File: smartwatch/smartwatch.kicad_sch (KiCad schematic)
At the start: 2 parts, among them U1 ESP32-S3-WROOM-1, U2 AMS1117-3.3

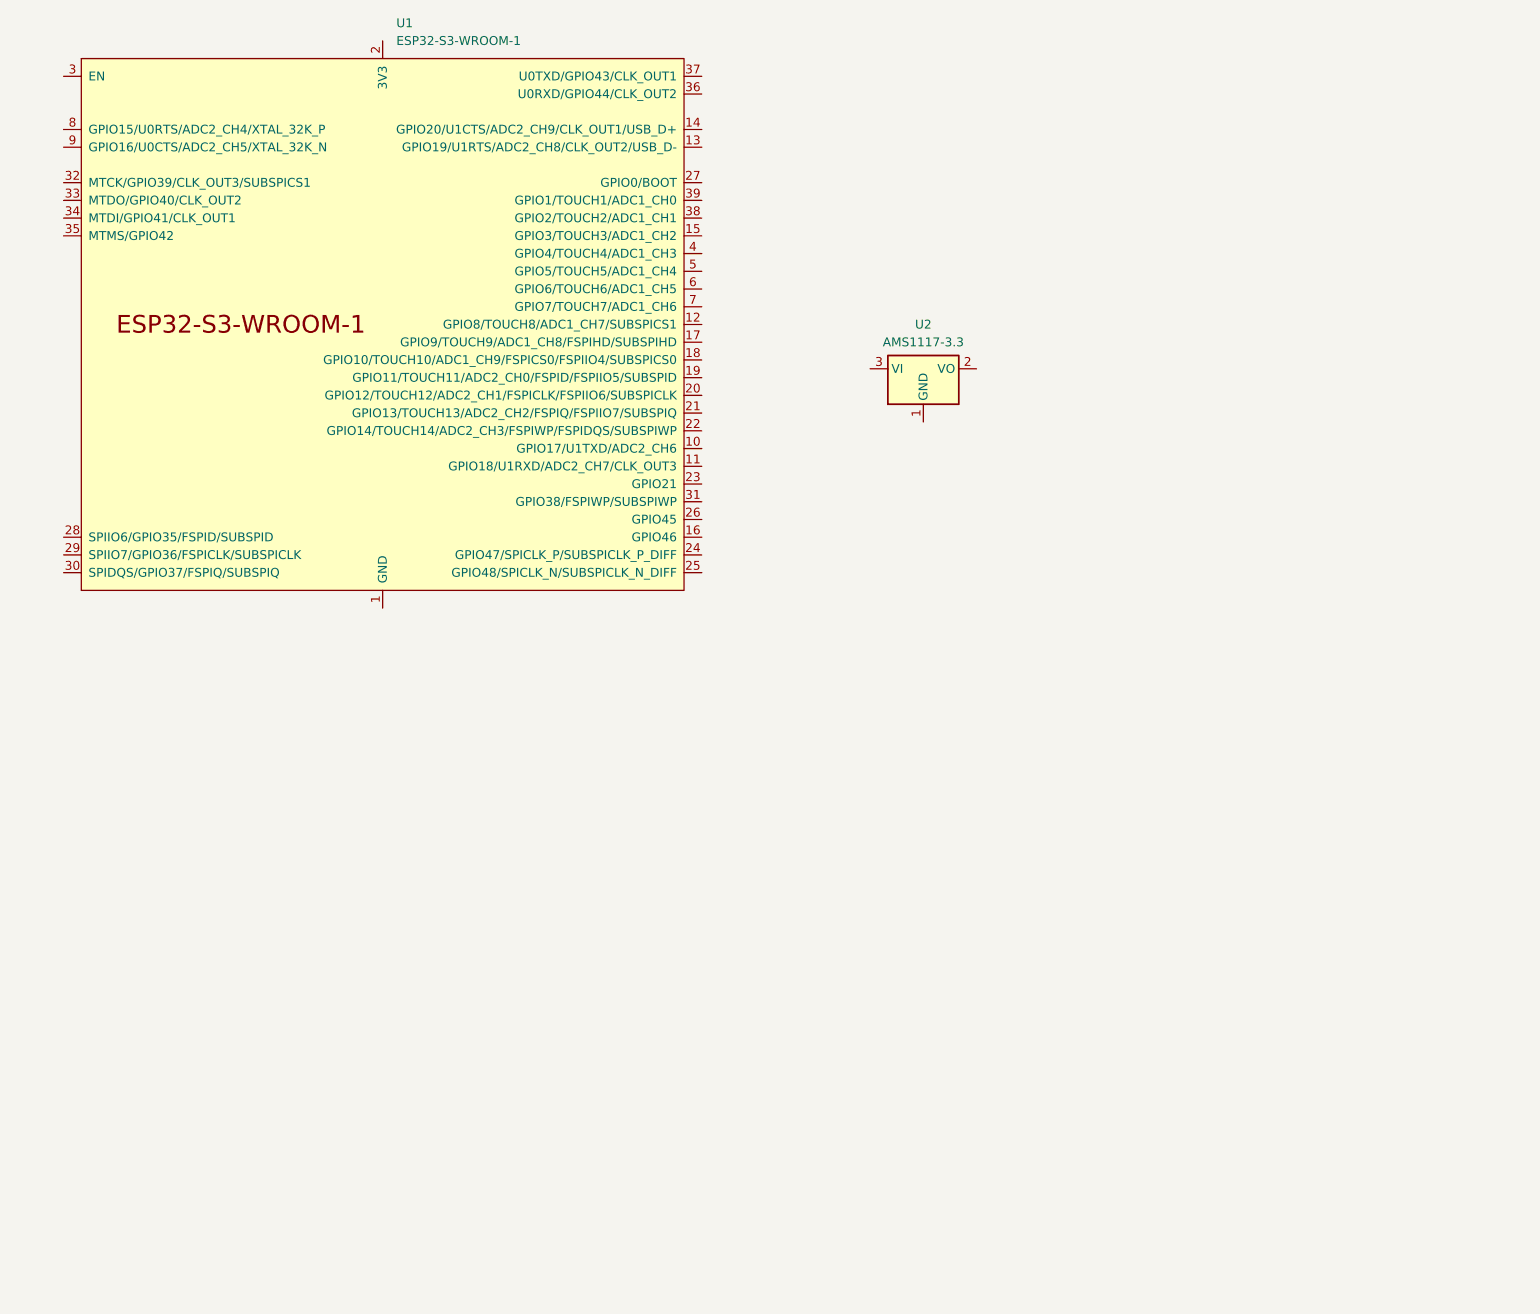
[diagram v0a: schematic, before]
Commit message: finished pcb and sch
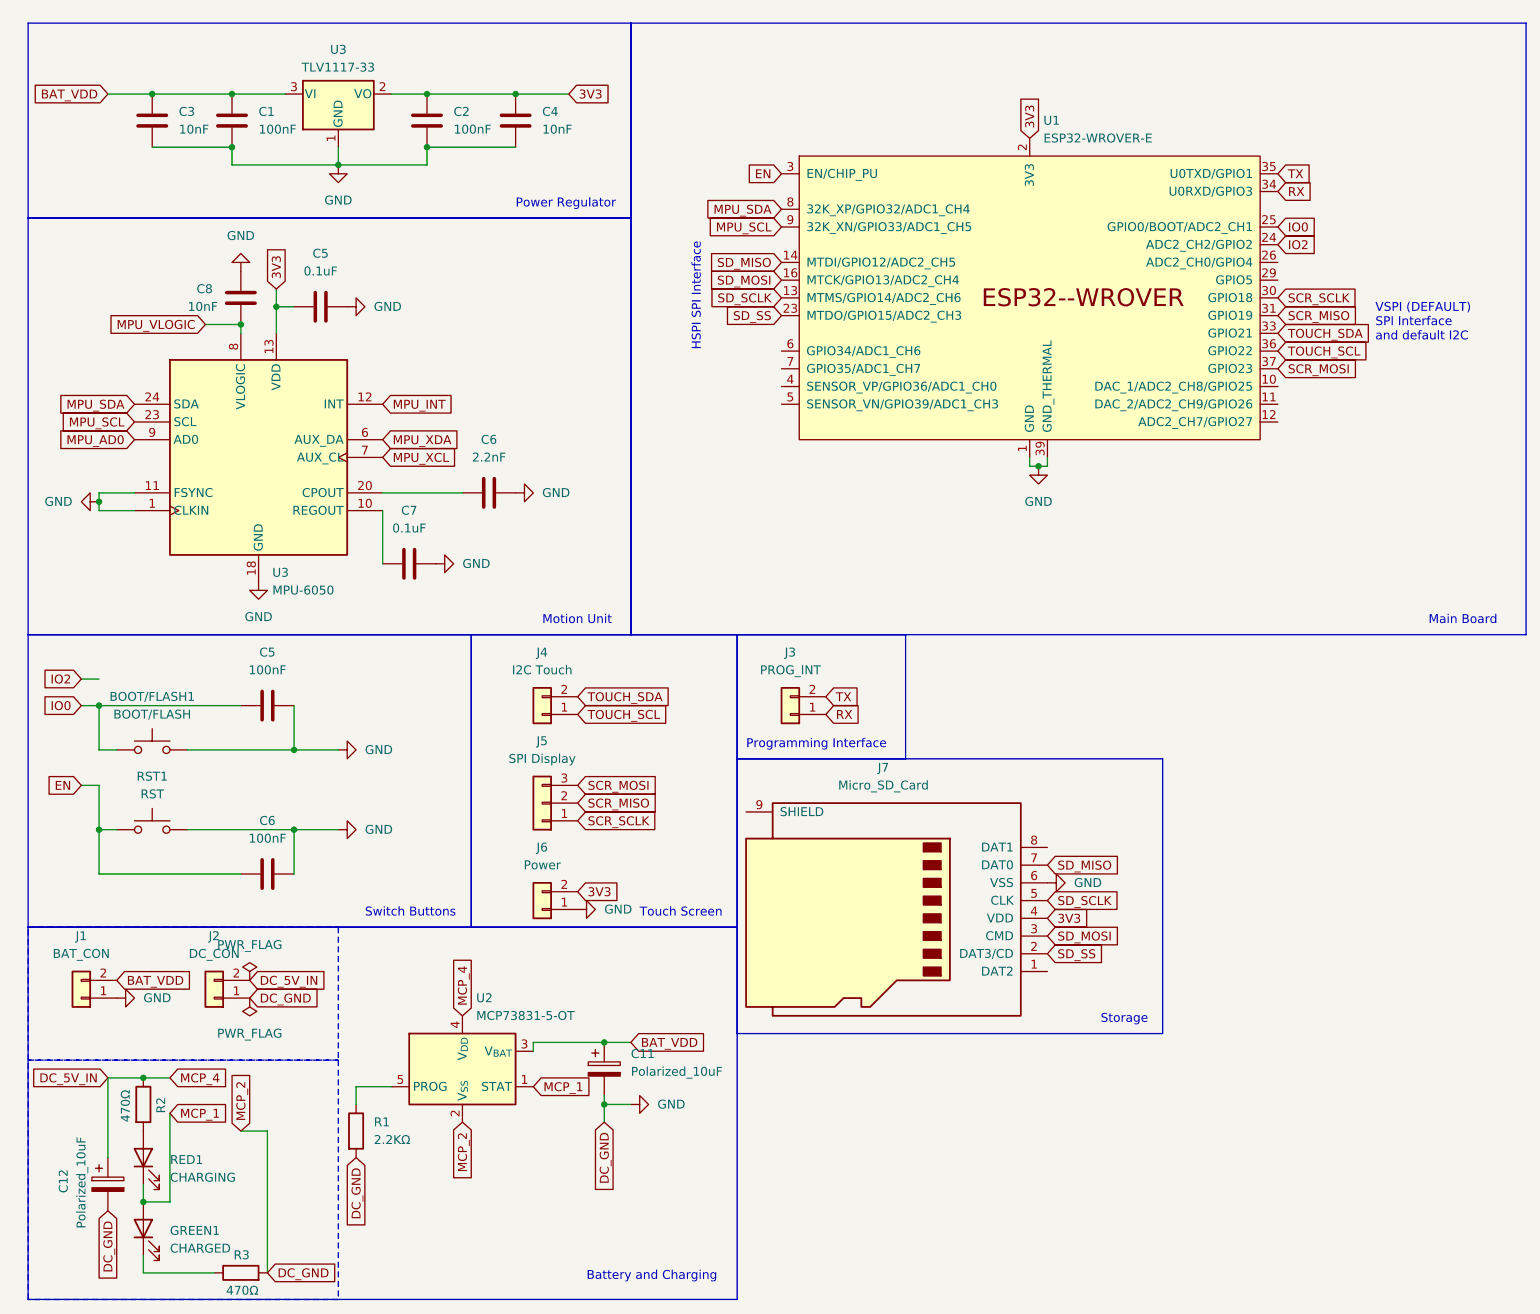
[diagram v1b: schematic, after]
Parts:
- removed U1: ESP32-S3-WROOM-1, Espressif:ESP32-WROVER-E, symbol Espressif:ESP32-S3-WROOM-1
- removed U2: AMS1117-3.3, Package_TO_SOT_SMD:SOT-223-3_TabPin2, symbol Regulator_Linear:AMS1117-3.3
- added BOOT/FLASH1: BOOT/FLASH, Button_Switch_SMD:SW_SPST_Omron_B3FS-100xP, symbol Switch:SW_Push
- added C1, C2, C5, C6: 100nF, Capacitor_SMD:C_0805_2012Metric_Pad1.18x1.45mm_HandSolder, symbol Device:C
- added C11, C12: Polarized_10uF, Capacitor_Tantalum_SMD:CP_EIA-2012-12_Kemet-R_Pad1.30x1.05mm_HandSolder, symbol Device:C_Polarized
- added C3, C4, C8: 10nF, Capacitor_SMD:C_0805_2012Metric_Pad1.18x1.45mm_HandSolder, symbol Device:C
- added C5, C7: 0.1uF, Capacitor_SMD:C_0805_2012Metric_Pad1.18x1.45mm_HandSolder, symbol Device:C
- added C6: 2.2nF, Capacitor_SMD:C_0805_2012Metric_Pad1.18x1.45mm_HandSolder, symbol Device:C
- added GREEN1: CHARGED, LED_SMD:LED_0805_2012Metric_Pad1.15x1.40mm_HandSolder, symbol Device:LED
- added J1: BAT_CON, Connector_Wire_SMD:Wire_Pad_1x02, symbol Connector_Generic:Conn_01x02
- added J2: DC_CON, Connector_Wire_SMD:Wire_Pad_1x02, symbol Connector_Generic:Conn_01x02
- added J3: PROG_INT, Connector_Wire_SMD:Wire_Pad_1x02, symbol Connector_Generic:Conn_01x02
- added J4: I2C Touch, Connector_Wire_SMD:Wire_Pad_1x02, symbol Connector_Generic:Conn_01x02
- added J5: SPI Display, Connector_Wire_SMD:Wire_Pad_1x03, symbol Connector_Generic:Conn_01x03
- added J6: Power, Connector_Wire_SMD:Wire_Pad_1x02, symbol Connector_Generic:Conn_01x02
- added J7: Micro_SD_Card, Connector_Card:microSD_HC_Hirose_DM3D-SF, symbol Connector:Micro_SD_Card
- added R1: 2.2KΩ, Resistor_SMD:R_0805_2012Metric_Pad1.20x1.40mm_HandSolder, symbol Device:R
- added R2, R3: 470Ω, Resistor_SMD:R_0805_2012Metric_Pad1.20x1.40mm_HandSolder, symbol Device:R
- added RED1: CHARGING, LED_SMD:LED_0805_2012Metric_Pad1.15x1.40mm_HandSolder, symbol Device:LED
- added RST1: RST, Button_Switch_SMD:SW_SPST_Omron_B3FS-100xP, symbol Switch:SW_Push
- added U1: ESP32-WROVER-E, Espressif:ESP32-WROVER-E, symbol Espressif:ESP32-WROVER-E
- added U2: MCP73831-5-OT, Package_TO_SOT_SMD:SOT-23-5, symbol Battery_Management:MCP73831-5-OT
- added U3: TLV1117-33, Package_TO_SOT_SMD:SOT-223-3_TabPin2, symbol Regulator_Linear:TLV1117-33
- added U3: MPU-6050, Sensor_Motion:InvenSense_QFN-24_4x4mm_P0.5mm, symbol Sensor_Motion:MPU-6050
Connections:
- new net: R2.2, RED1.2 (A)
- new net: C7.1, U3.10 (REGOUT)
- new net: C6.1, U3.20 (CPOUT)
- new net: GREEN1.1 (K), R3.1
- new net: R1.1, U2.5 (PROG)
- new net 3V3: C2.2, C4.2, C5.1, J6.2 (Pin_2), J7.4 (VDD), U1.2 (3V3), U3.13 (VDD), U3.2 (VO)
- new net BAT_VDD: C1.2, C11.1, C3.2, J1.2 (Pin_2), U2.3 (V_{BAT}), U3.3 (VI)
- new net DC_5V_IN: C12.1, J2.2 (Pin_2), R2.1, U2.4 (V_{DD})
- new net EN: C6.2, RST1.1, U1.3 (EN/CHIP_PU)
- new net GND: BOOT/FLASH1.2, C1.1, C11.2, C12.2, C2.1, C3.1, C4.1, C5.1, C5.2, C6.1, C6.2, C7.2, C8.2, J1.1 (Pin_1), J2.1 (Pin_1), J6.1 (Pin_1), J7.6 (VSS), R1.2, R3.2, RST1.2, U1.1 (GND), U1.15 (GND), U1.38 (GND), U1.39 (GND_THERMAL), U2.2 (V_{SS}), U3.1 (CLKIN), U3.1 (GND), U3.11 (FSYNC), U3.18 (GND)
- new net IO0: BOOT/FLASH1.1, C5.2, U1.25 (GPIO0/BOOT/ADC2_CH1)
- new net IO2: U1.24 (ADC2_CH2/GPIO2)
- new net MCP_1: GREEN1.2 (A), RED1.1 (K), U2.1 (STAT)
- new net MPU_AD0: U3.9 (AD0)
- new net MPU_INT: U3.12 (INT)
- new net MPU_SCL: U1.9 (32K_XN/GPIO33/ADC1_CH5), U3.23 (SCL)
- new net MPU_SDA: U1.8 (32K_XP/GPIO32/ADC1_CH4), U3.24 (SDA)
- new net MPU_VLOGIC: C8.1, U3.8 (VLOGIC)
- new net MPU_XCL: U3.7 (AUX_CL)
- new net MPU_XDA: U3.6 (AUX_DA)
- new net RX: J3.1 (Pin_1), U1.34 (U0RXD/GPIO3)
- new net SCR_MISO: J5.2 (Pin_2), U1.31 (GPIO19)
- new net SCR_MOSI: J5.3 (Pin_3), U1.37 (GPIO23)
- new net SCR_SCLK: J5.1 (Pin_1), U1.30 (GPIO18)
- new net SD_MISO: J7.7 (DAT0), U1.14 (MTDI/GPIO12/ADC2_CH5)
- new net SD_MOSI: J7.3 (CMD), U1.16 (MTCK/GPIO13/ADC2_CH4)
- new net SD_SCLK: J7.5 (CLK), U1.13 (MTMS/GPIO14/ADC2_CH6)
- new net SD_SS: J7.2 (DAT3/CD), U1.23 (MTDO/GPIO15/ADC2_CH3)
- new net TOUCH_SCL: J4.1 (Pin_1), U1.36 (GPIO22)
- new net TOUCH_SDA: J4.2 (Pin_2), U1.33 (GPIO21)
- new net TX: J3.2 (Pin_2), U1.35 (U0TXD/GPIO1)
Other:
- note added: "Battery and Charging"
- note added: "HSPI SPI Interface"
- note added: "Main Board"
- note added: "Motion Unit"
- note added: "Power Regulator"
- note added: "Programming Interface"
- note added: "Storage"
- note added: "Switch Buttons"
- note added: "Touch Screen"
- note added: "VSPI (DEFAULT) SPI Interface and default I2C"
